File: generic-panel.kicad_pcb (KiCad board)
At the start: 2 copper layers, 85 x 98.6 mm, 182 parts, among them J1 CONN_6, J3 RCA, J4 Mini-DIN-4, J5 Conn_01x04_Male, U1 AD724, Y1 4.433619M

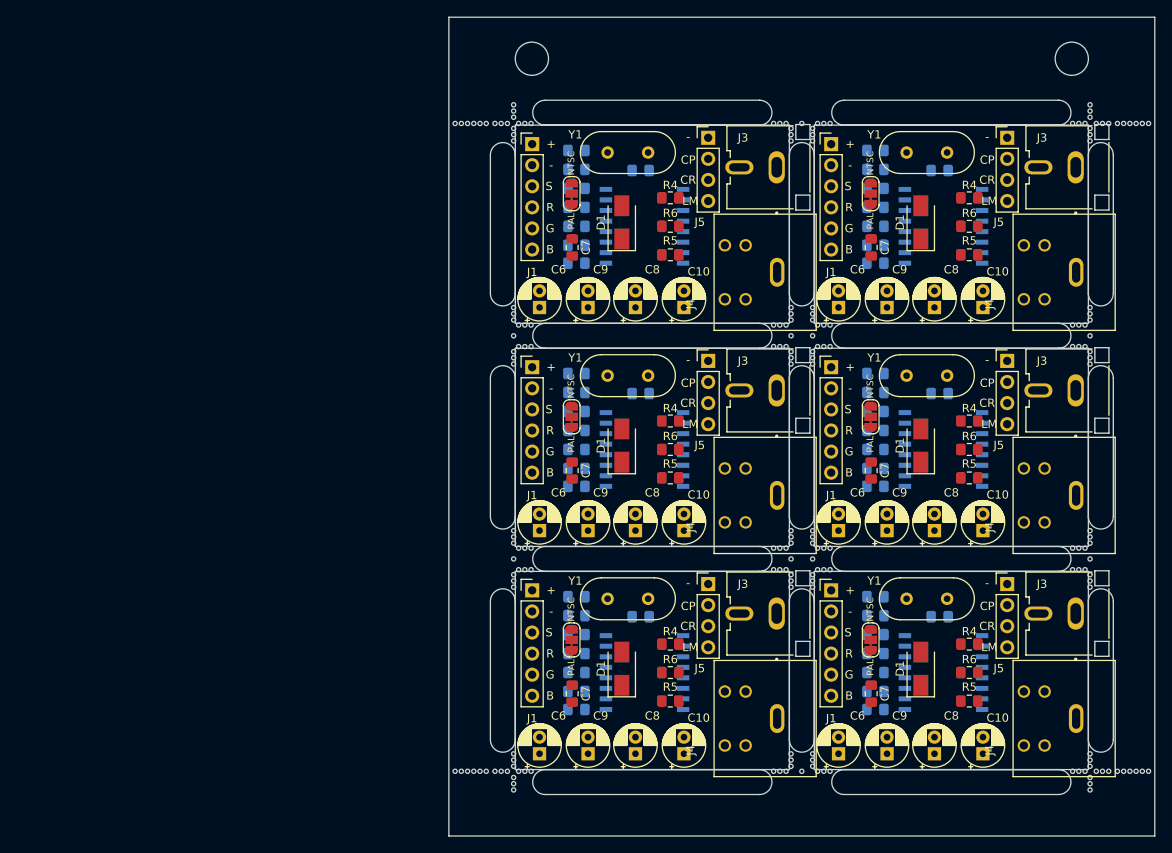
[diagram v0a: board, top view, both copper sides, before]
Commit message: release candidate
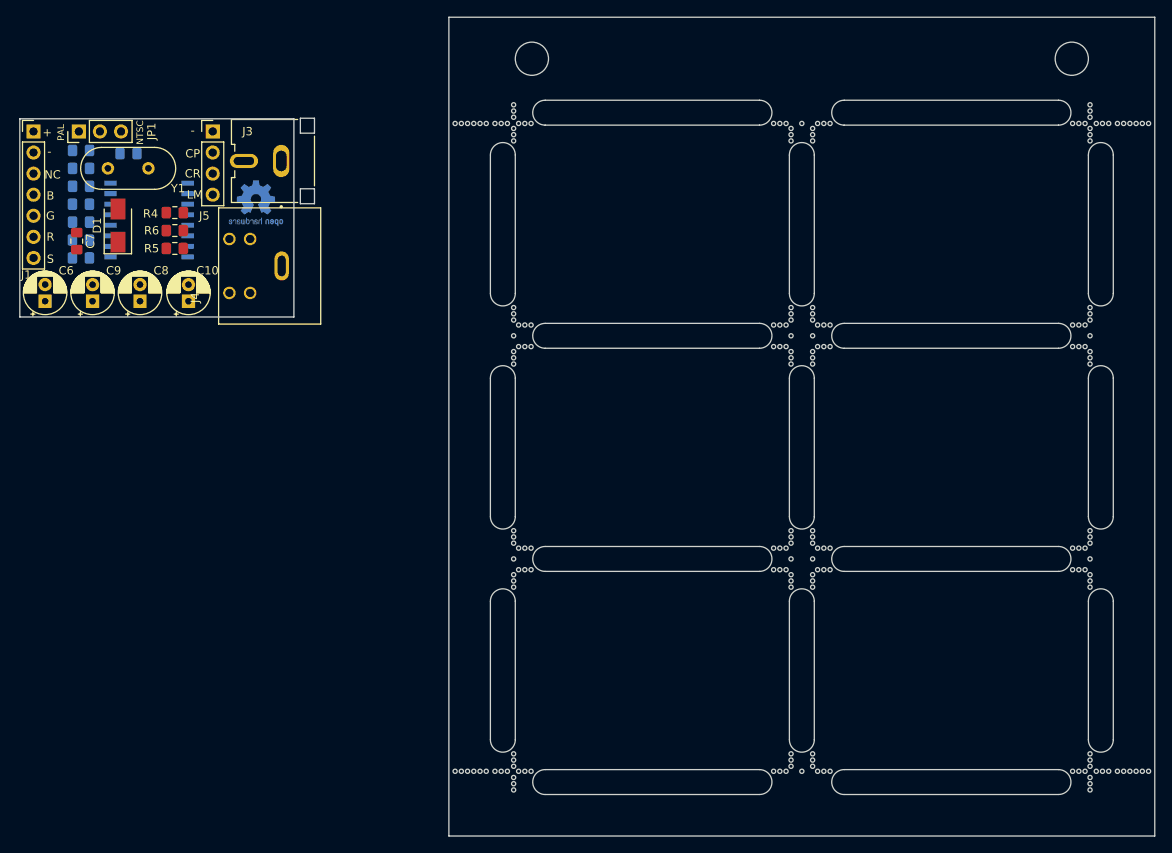
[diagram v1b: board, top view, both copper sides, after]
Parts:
- removed the C1 at (43.4, 56.8)
- removed the C1 at (7.37, 56.8)
- removed the C1 at (43.4, 29.9)
- removed the C1 at (7.37, 29.9)
- removed the C1 at (43.4, 3.05)
- removed the C10 at (56.3, 75.7)
- removed the C10 at (20.3, 75.7)
- removed the C10 at (56.3, 48.9)
- removed the C10 at (20.3, 48.9)
- removed the C10 at (56.3, 22.0)
- removed the C2 at (43.4, 68.2)
- removed the C2 at (7.36, 68.2)
- removed the C2 at (43.4, 41.4)
- removed the C2 at (7.36, 41.4)
- removed the C2 at (43.4, 14.5)
- removed the C3 at (43.4, 63.7)
- removed the C3 at (7.37, 63.7)
- removed the C3 at (43.4, 36.8)
- removed the C3 at (7.37, 36.8)
- removed the C3 at (43.4, 9.91)
- removed the C4 at (43.4, 59.1)
- removed the C4 at (7.37, 59.1)
- removed the C4 at (43.4, 32.2)
- removed the C4 at (7.37, 32.2)
- removed the C4 at (43.4, 5.33)
- removed the C5 at (51.1, 59.2)
- removed the C5 at (15.1, 59.2)
- removed the C5 at (51.1, 32.3)
- removed the C5 at (15.1, 32.3)
- removed the C5 at (51.1, 5.46)
- removed the C5 at (15.1, 5.46)
- removed the C6 at (38.9, 75.7)
- removed the C6 at (2.92, 75.7)
- removed the C6 at (38.9, 48.9)
- removed the C6 at (2.92, 48.9)
- removed the C6 at (38.9, 22.0)
- removed the C7 at (42.9, 68.5)
- removed the C7 at (6.86, 68.5)
- removed the C7 at (42.9, 41.6)
- removed the C7 at (6.86, 41.6)
- removed the C7 at (42.9, 14.7)
- removed the C8 at (50.5, 75.7)
- removed the C8 at (14.5, 75.7)
- removed the C8 at (50.5, 48.9)
- removed the C8 at (14.5, 48.9)
- removed the C8 at (50.5, 22.0)
- removed the C9 at (44.8, 75.7)
- removed the C9 at (8.76, 75.7)
- removed the C9 at (44.8, 48.9)
- removed the C9 at (8.76, 48.9)
- removed the C9 at (44.8, 22.0)
- removed the D1 at (48.8, 65.5)
- removed the D1 at (12.8, 65.5)
- removed the D1 at (48.8, 38.6)
- removed the D1 at (12.8, 38.6)
- removed the D1 at (48.8, 11.7)
- removed the J1 at (38.1, 56.0)
- removed the J1 at (2.03, 56.0)
- removed the J1 at (38.1, 29.2)
- removed the J1 at (2.03, 29.2)
- removed the J1 at (38.1, 2.29)
- removed the J1 at (2.03, 2.29)
- removed the J3 at (67.5, 58.8)
- removed the J3 at (31.5, 58.8)
- removed the J3 at (67.5, 32.0)
- removed the J3 at (31.5, 32.0)
- removed the J3 at (67.5, 5.08)
- removed the J4 at (66.1, 71.5)
- removed the J4 at (30.1, 71.5)
- removed the J4 at (66.1, 44.6)
- removed the J4 at (30.1, 44.6)
- removed the J4 at (66.1, 17.7)
- removed the J5 at (59.3, 55.3)
- removed the J5 at (23.2, 55.3)
- removed the J5 at (59.3, 28.4)
- removed the J5 at (23.2, 28.4)
- removed the J5 at (59.3, 1.52)
- removed the JP1 at (42.8, 62.0)
- removed the JP1 at (6.79, 62.0)
- removed the JP1 at (42.8, 35.1)
- removed the JP1 at (6.79, 35.1)
- removed the JP1 at (42.8, 8.26)
- removed the R1 at (43.4, 70.4)
- removed the R1 at (7.36, 70.4)
- removed the R1 at (43.4, 43.5)
- removed the R1 at (7.36, 43.5)
- removed the R1 at (43.4, 16.6)
- removed the R2 at (43.4, 66.0)
- removed the R2 at (7.37, 66.0)
- removed the R2 at (43.4, 39.1)
- removed the R2 at (7.37, 39.1)
- removed the R2 at (43.4, 12.2)
- removed the R3 at (43.4, 61.4)
- removed the R3 at (7.38, 61.4)
- removed the R3 at (43.4, 34.5)
- removed the R3 at (7.38, 34.5)
- removed the R3 at (43.4, 7.62)
- removed the R4 at (54.7, 62.5)
- removed the R4 at (18.7, 62.5)
- removed the R4 at (54.7, 35.6)
- removed the R4 at (18.7, 35.6)
- removed the R4 at (54.7, 8.76)
- removed the R5 at (54.7, 69.4)
- removed the R5 at (18.7, 69.4)
- removed the R5 at (54.7, 42.5)
- removed the R5 at (18.7, 42.5)
- removed the R5 at (54.7, 15.6)
- removed the R6 at (54.7, 66.0)
- removed the R6 at (18.7, 66.0)
- removed the R6 at (54.7, 39.1)
- removed the R6 at (18.7, 39.1)
- removed the R6 at (54.7, 12.2)
- removed the U1 at (51.6, 66.0)
- removed the U1 at (15.6, 66.0)
- removed the U1 at (51.6, 39.1)
- removed the U1 at (15.6, 39.1)
- removed the U1 at (51.6, 12.2)
- removed the U1 at (15.6, 12.2)
- removed the Y1 at (52.0, 57.1)
- removed the Y1 at (16.0, 57.1)
- removed the Y1 at (52.0, 30.2)
- removed the Y1 at (16.0, 30.2)
- removed the Y1 at (52.0, 3.30)
- added C5: 100n, Capacitor_SMD:C_0805_2012Metric_Pad1.15x1.40mm_HandSolder, B.Cu at (-46.6, 3.43)
- added J1: CONN_7, Connector_PinHeader_2.54mm:PinHeader_1x07_P2.54mm_Vertical, F.Cu at (-58.0, 0.76)
- added P1: OSHW_LOGO, Symbol:OSHW-Logo2_7.3x6mm_Copper, B.Cu at (-31.2, 9.40)
- added U1: AD724, Package_SO:SOIC-16W_7.5x10.3mm_P1.27mm, B.Cu at (-44.1, 11.4)
- JP1: footprint OpenVideoModulator:SolderJumper-3_P1.3mm_Bridged12_RoundedPad1.0x1.5mm -> Connector_PinHeader_2.54mm:PinHeader_1x03_P2.54mm_Vertical
- moved D1 60.7 mm to (-47.9, 12.1)
- moved Y1 60.2 mm to (-44.2, 5.21)
- moved JP1 59.8 mm to (-52.6, 0.76)
- moved R4 59.7 mm to (-41.0, 10.5)
- moved C8 59.7 mm to (-45.2, 21.2)
- moved C10 59.7 mm to (-39.4, 21.2)
- moved C7 59.7 mm to (-52.8, 14.0)
- moved C9 59.7 mm to (-50.9, 21.2)
- moved J3 59.7 mm to (-28.2, 4.32)
- moved J4 59.7 mm to (-29.6, 17.0)
- moved J5 59.7 mm to (-36.4, 0.76)
- moved R5 59.7 mm to (-41.0, 14.9)
- moved C2 59.7 mm to (-52.3, 13.8)
- moved R1 59.7 mm to (-52.3, 16.0)
- moved R6 59.7 mm to (-41.0, 12.7)
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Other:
- board size 85 x 98.6 mm -> 136.7 x 98.6 mm
- board text added: "NC"
- board text added: "github.com/ issalig/ OpenVideo Modulator"
- board text removed: "github.com/issalig/OpenVideoModulator"
